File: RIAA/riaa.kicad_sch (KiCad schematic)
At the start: 48 parts, among them J1 Conn_01x04_Socket, J2 Conn_01x04_Socket, J3 Conn_01x04_Socket, Q1 2N2222, Q10 2N2222, Q11 2N2222, Q12 2N2907, Q13 2N2907, Q14 2N2222, Q2 2N2222, Q3 2N2222, Q4 2N2222, Q5 2N2907, Q6 2N2907, Q7 2N2907, Q8 2N2907, Q9 2N2222, U105 TL072

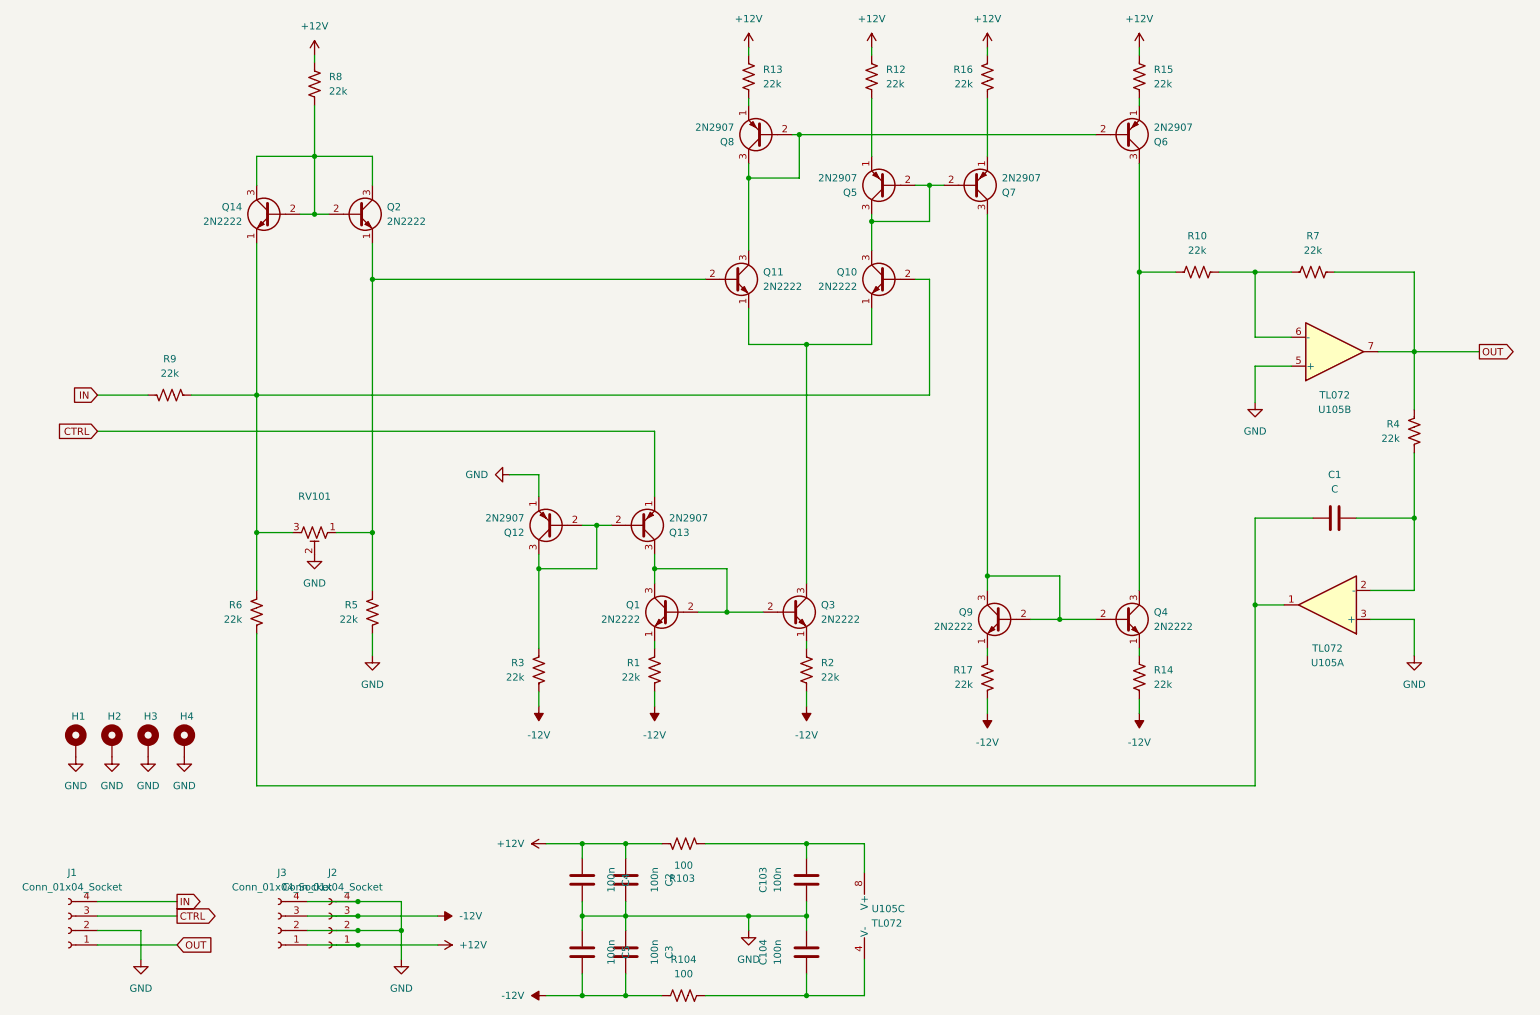
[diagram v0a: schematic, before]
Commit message: v1
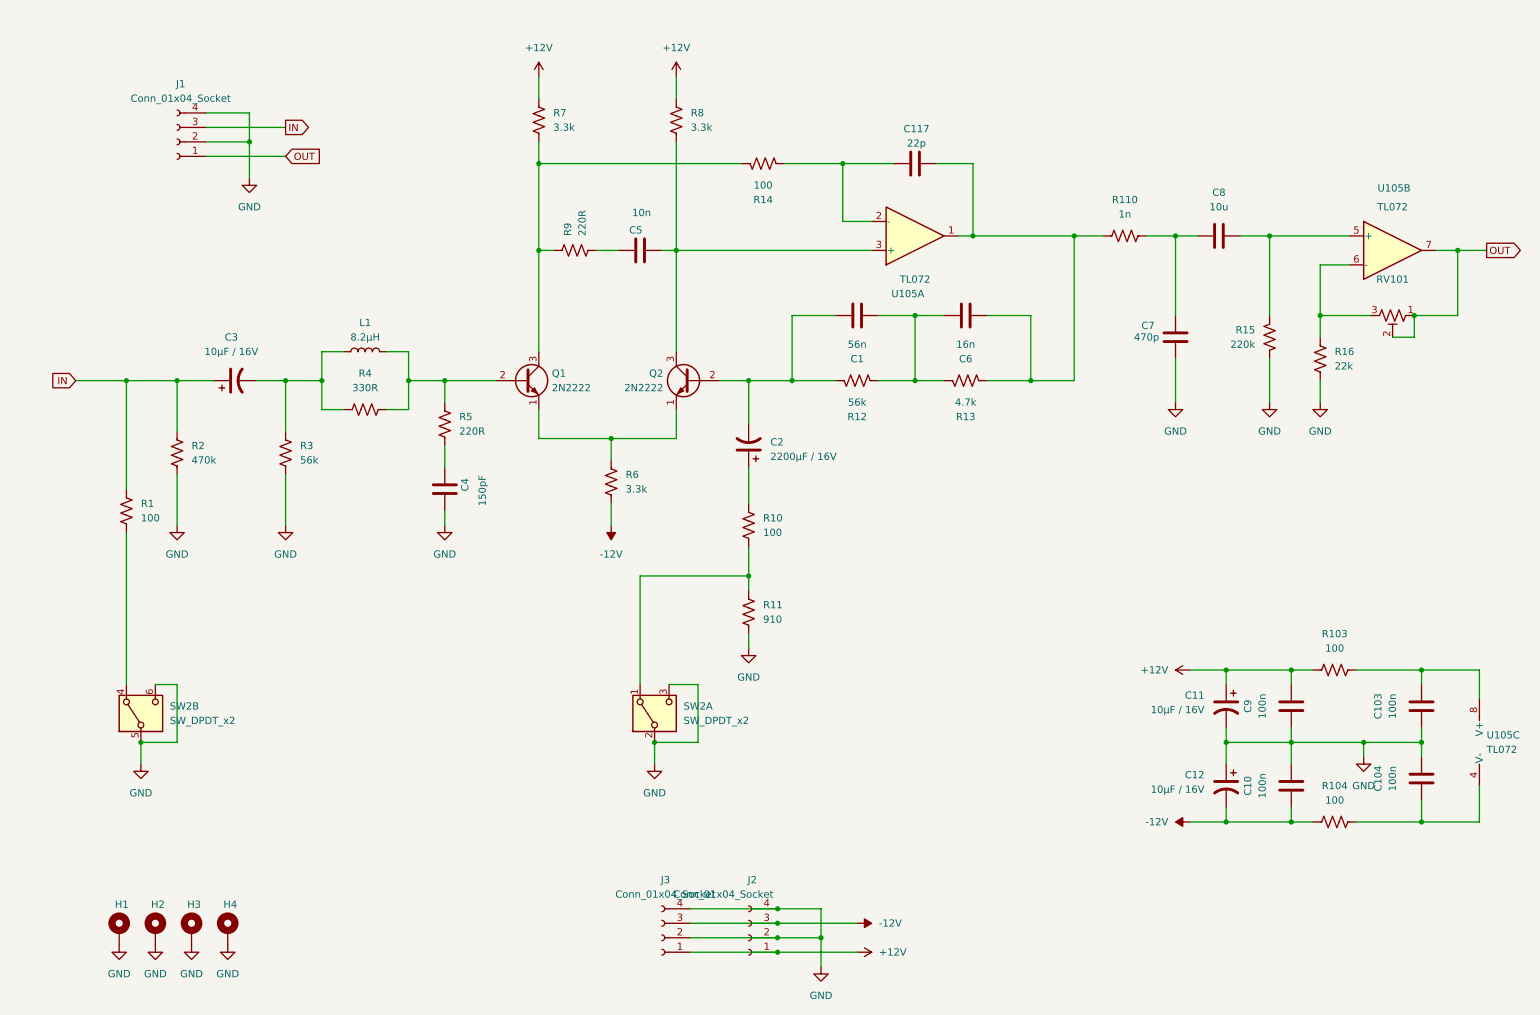
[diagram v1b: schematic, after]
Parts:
- removed C2, C3: 100n, Capacitor_THT:C_Disc_D4.3mm_W1.9mm_P5.00mm, symbol Device:C
- removed Q10, Q11, Q14, Q3, Q4, Q9: 2N2222, Package_TO_SOT_THT:TO-46-3, symbol Transistor_BJT:Q_NPN_EBC
- removed Q12, Q13, Q5, Q6, Q7, Q8: 2N2907, Package_TO_SOT_THT:TO-46-3, symbol Transistor_BJT:Q_PNP_EBC
- removed R17: 22k, Resistor_THT:R_Axial_DIN0207_L6.3mm_D2.5mm_P10.16mm_Horizontal, symbol Device:R_US
- added C10, C9: 100n, Capacitor_THT:C_Disc_D4.3mm_W1.9mm_P5.00mm, symbol Device:C
- added C11, C12, C3: 10µF / 16V, Capacitor_THT:CP_Radial_D8.0mm_P2.50mm, symbol Device:C_Polarized_US
- added C117: 22p, Capacitor_THT:C_Disc_D4.3mm_W1.9mm_P5.00mm, symbol Device:C
- added C2: 2200µF / 16V, Capacitor_THT:CP_Radial_D8.0mm_P2.50mm, symbol Device:C_Polarized_US
- added C6: 16n, Capacitor_THT:C_Disc_D4.3mm_W1.9mm_P5.00mm, symbol Device:C
- added C7: 470p, Capacitor_THT:C_Disc_D4.3mm_W1.9mm_P5.00mm, symbol Device:C
- added C8: 10u, Capacitor_THT:C_Disc_D9.0mm_W5.0mm_P5.00mm, symbol Device:C
- added L1: 8.2µH, Inductor_THT:L_Axial_L9.5mm_D4.0mm_P12.70mm_Horizontal_Fastron_SMCC, symbol Device:L
- added R11: 910, Resistor_THT:R_Axial_DIN0207_L6.3mm_D2.5mm_P10.16mm_Horizontal, symbol Device:R_US
- added R110: 1n, Resistor_THT:R_Axial_DIN0207_L6.3mm_D2.5mm_P10.16mm_Horizontal, symbol Device:R_US
- added SW2: SW_DPDT_x2, Button_Switch_THT:SW_PUSH_E-Switch_FS5700DP_DPDT, symbol Switch:SW_DPDT_x2
- C1: value C -> 56n; footprint Capacitor_THT:C_Disc_D9.0mm_W5.0mm_P5.00mm -> Capacitor_THT:C_Disc_D4.3mm_W1.9mm_P5.00mm
- C4: value 100n -> 150pF
- C5: value 100n -> 10n
- R1, R10, R14: value 22k -> 100
- R12, R3: value 22k -> 56k
- R13: value 22k -> 4.7k
- R15: value 22k -> 220k
- R2: value 22k -> 470k
- R4: value 22k -> 330R
- R5, R9: value 22k -> 220R
- R6, R7, R8: value 22k -> 3.3k
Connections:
- net CTRL is gone; now on net IN: J1.3 (Pin_3)
- net +12V: now also R7.1, C11.1, C9.2; no longer C4.2, R12.1, R13.1, R15.1, R16.1
- net -12V: now also R6.2, C10.1, C12.2; no longer C5.1, R1.2, R14.2, R2.2, R3.2
- net GND: now also J1.4 (Pin_4), R15.2, R16.2, R2.2, R3.2, C10.2, C11.2, C12.1, C7.2, C9.1, R11.2, SW2.2 (B), SW2.3 (C), SW2.5 (B), SW2.6 (C); no longer C5.2, R5.2, RV101.2, U105.3 (+), U105.5 (+)
- net IN: now also R1.1, R2.1, C3.1; no longer J1.4 (Pin_4), R9.1
- net OUT: now also RV101.1, RV101.2; no longer R4.1, R7.2
- net at R12.2: now also C1.1, R13.1, C6.2
- net at R13.2: now also U105.1, C117.2, C6.1, R110.2
- net at R3.1: now also R4.1, C3.2, L1.1
- net at Q1.2 (B): now also R4.2, R5.1, L1.2; no longer Q1.3 (C)
- net at Q1.1 (E): now also Q2.1 (E), R6.1; no longer R1.1
- net at Q2.3 (C), R8.2: now also C5.1, U105.3 (+); no longer Q2.2 (B)
- net at R10.1: now also C2.1
- net at R14.1: now also Q1.3 (C), R7.2, R9.1
- new net: C8.1, R15.1, U105.5 (+)
- new net: R1.2, SW2.4 (A)
- new net: C7.1, C8.2, R110.1
- new net: C4.2, R5.2
- new net: R16.1, RV101.3, U105.6 (-)
- new net: C117.1, R14.2, U105.2 (-)
- new net: C1.2, C2.2, Q2.2 (B), R12.1
- new net: R10.2, R11.1, SW2.1 (A)
- new net: C5.2, R9.2
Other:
- moved on the sheet: C103, C104, H1, H2, H3, H4, J1, J2, R103, R104, RV101
